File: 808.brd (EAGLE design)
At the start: 160 x 100 mm, 56 parts, among them IC1 TL072D, T1 BC846, T2 BC846, T3 BC846, T5 BC846, T6 BC846

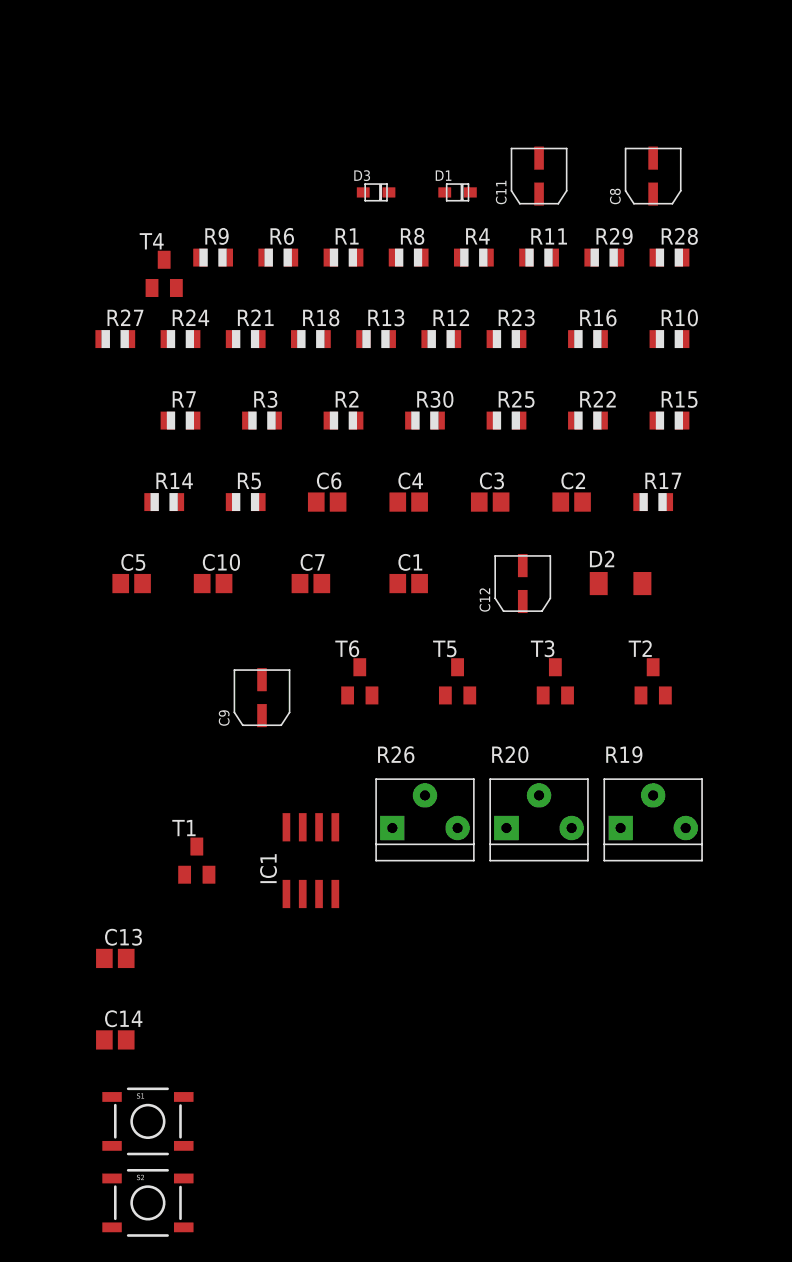
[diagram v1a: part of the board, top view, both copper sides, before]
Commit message: regenerating brd
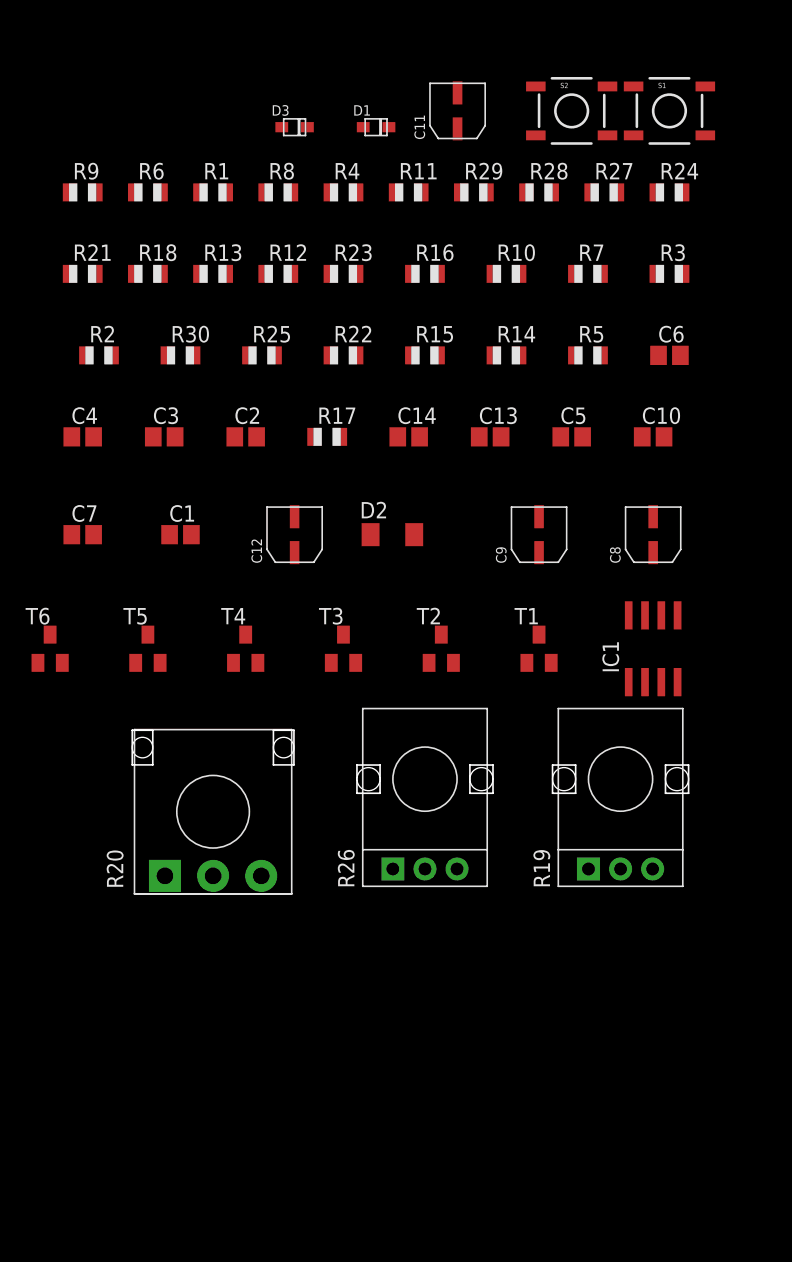
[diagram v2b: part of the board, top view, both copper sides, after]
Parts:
- C8: value 0.47uF -> 0.47uF / 50v
- R19: value 10k -> 10k Log; device 808:POTENTIOMETER-3352P -> 808:POTENTIOMETER-PTV09
- R20: value 10k -> 100k Lin; device 808:POTENTIOMETER-3352P -> 808:POTENTIOMETER-CTS296
- R26: value 500k -> 500k Lin; device 808:POTENTIOMETER-3352P -> 808:POTENTIOMETER-PTV09
- T4: value (none) -> BC856
- moved S2 91.3 mm to (-24.1, 62.2)
- moved S1 88.6 mm to (-16.5, 62.2)
- moved C14 52.3 mm to (-36.8, 36.8)
- moved C13 50.0 mm to (-30.5, 36.8)
- moved R24 39.8 mm to (-16.5, 55.9)
- moved R27 39.8 mm to (-21.6, 55.9)
- moved C5 36.1 mm to (-24.1, 36.8)
- moved C10 36.1 mm to (-17.8, 36.8)
- moved R3 33.7 mm to (-16.5, 49.5)
- moved R7 33.7 mm to (-22.9, 49.5)
- moved IC1 31.4 mm to (-17.8, 20.3)
- moved T1 31.4 mm to (-26.7, 20.3)
- moved T4 29.9 mm to (-49.5, 20.3)
- moved R14 29.0 mm to (-29.2, 43.2)
- moved R5 29.0 mm to (-22.9, 43.2)
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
